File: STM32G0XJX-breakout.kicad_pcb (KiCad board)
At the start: 4 copper layers, 10.5 x 11.5 mm, 5 parts, among them J1 PinHeader 1x4 2.54mm, J2 PinHeader 1x4 2.54mm, U1 STM32C011J6Mx

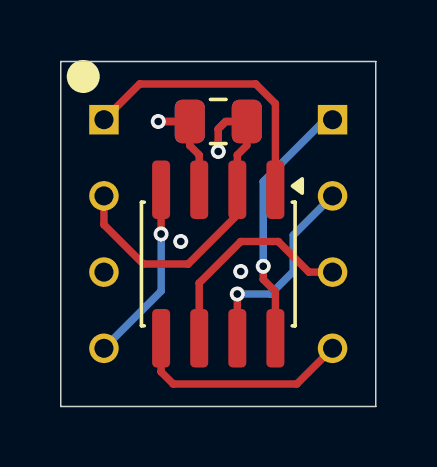
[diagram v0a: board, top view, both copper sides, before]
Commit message: done
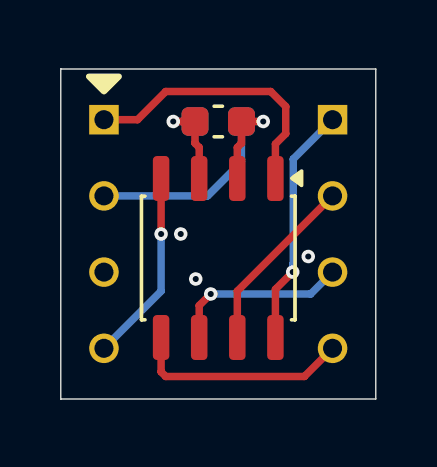
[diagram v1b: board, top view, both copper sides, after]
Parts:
- removed U1: STM32C011J6Mx, Package_SO:SOIC-8_3.9x4.9mm_P1.27mm
- added G***: LOGO, User_Graphics:Gort_Tech_2_Silk, B.Cu at (150.2, 102.8)
- added U2: STM32G031J6Mx, Package_SO:JEITA_SOIC-8_3.9x4.9mm_P1.27mm, F.Cu at (150.0, 100.8)
- C1: value 100n -> 2u2; footprint Capacitor_SMD:C_0805_2012Metric -> Capacitor_SMD:C_0603_1608Metric
- C2: value 4u7 -> 2u2; footprint Capacitor_SMD:C_0805_2012Metric -> Capacitor_SMD:C_0603_1608Metric
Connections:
- J1 pad 1: /PB7/PC14 -> /PB7/PB8/PB9/PC14
- J2 pad 1: /PA14/PB6/PC15 -> /PA14/PA15/PB5/PB6
- J2 pad 4: /PA8/PA9/PA11 -> /PA8/PA9/PA11/PB0/PB1
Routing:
- net /PB7/PC14: track 9.35 -> 0.00 mm
- net /PB7/PB8/PB9/PC14: track 0.00 -> 9.20 mm
- net /PA14/PB6/PC15: track 8.56 -> 0.00 mm, vias 1 -> 0
- net /PA14/PA15/PB5/PB6: track 0.00 -> 8.05 mm, vias 0 -> 1
- net /PA8/PA9/PA11: track 7.50 -> 0.00 mm
- net /PA8/PA9/PA11/PB0/PB1: track 0.00 -> 7.31 mm
- net +3.3V: track 13.5 -> 9.81 mm
- net /PA10/PA12: track 7.28 -> 5.97 mm, vias 0 -> 1
- net GND: track 4.51 -> 3.41 mm, vias 3 -> 4
- net /PA13: track 6.71 -> 6.04 mm, vias 1 -> 0
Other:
- board size 10.5 x 11.5 mm -> 10.5 x 11 mm
